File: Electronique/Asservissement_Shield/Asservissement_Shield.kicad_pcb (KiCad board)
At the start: 2 copper layers, 49 parts, among them J1 Hall_Sensor, J2 Windings, J3 Hall_Sensor, J4 Windings, P1 encoder_2, P2 encoder_2, U1 TXS0108EPW, U2 L6235PD, U3 L6235PD

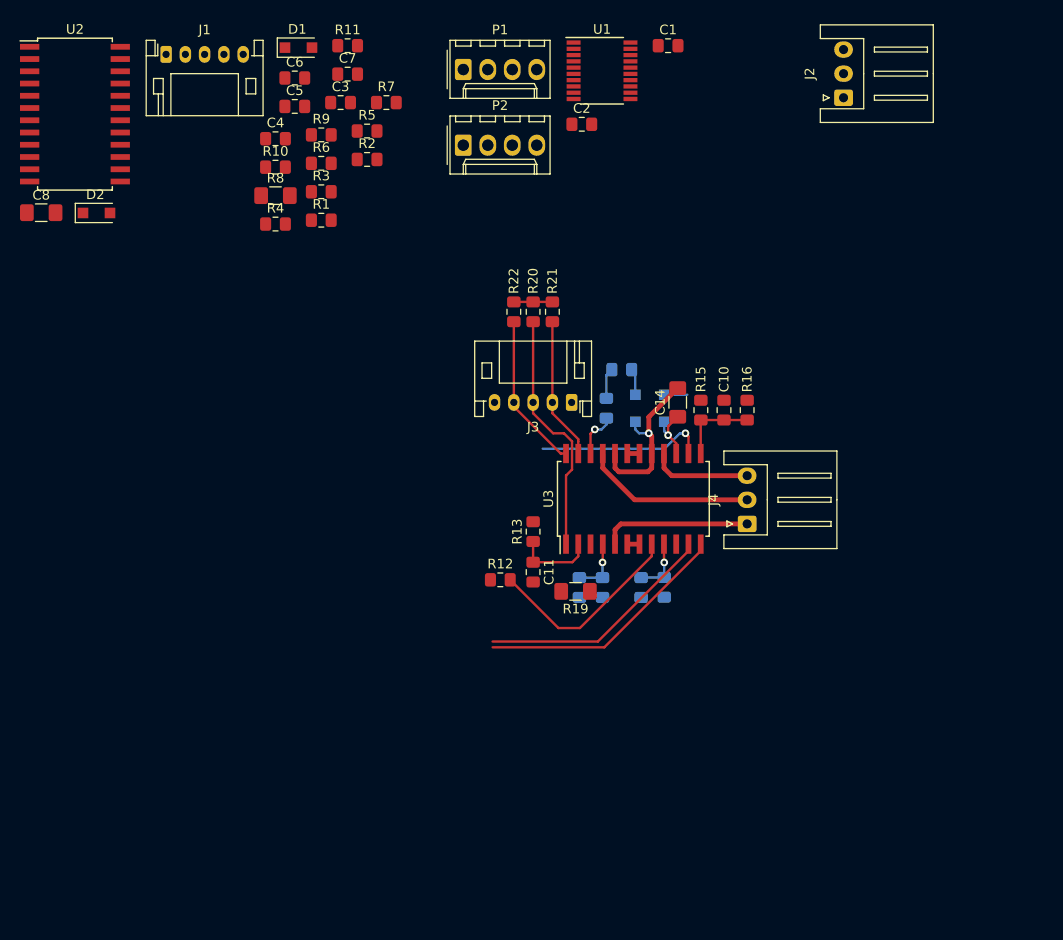
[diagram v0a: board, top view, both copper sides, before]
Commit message: oops
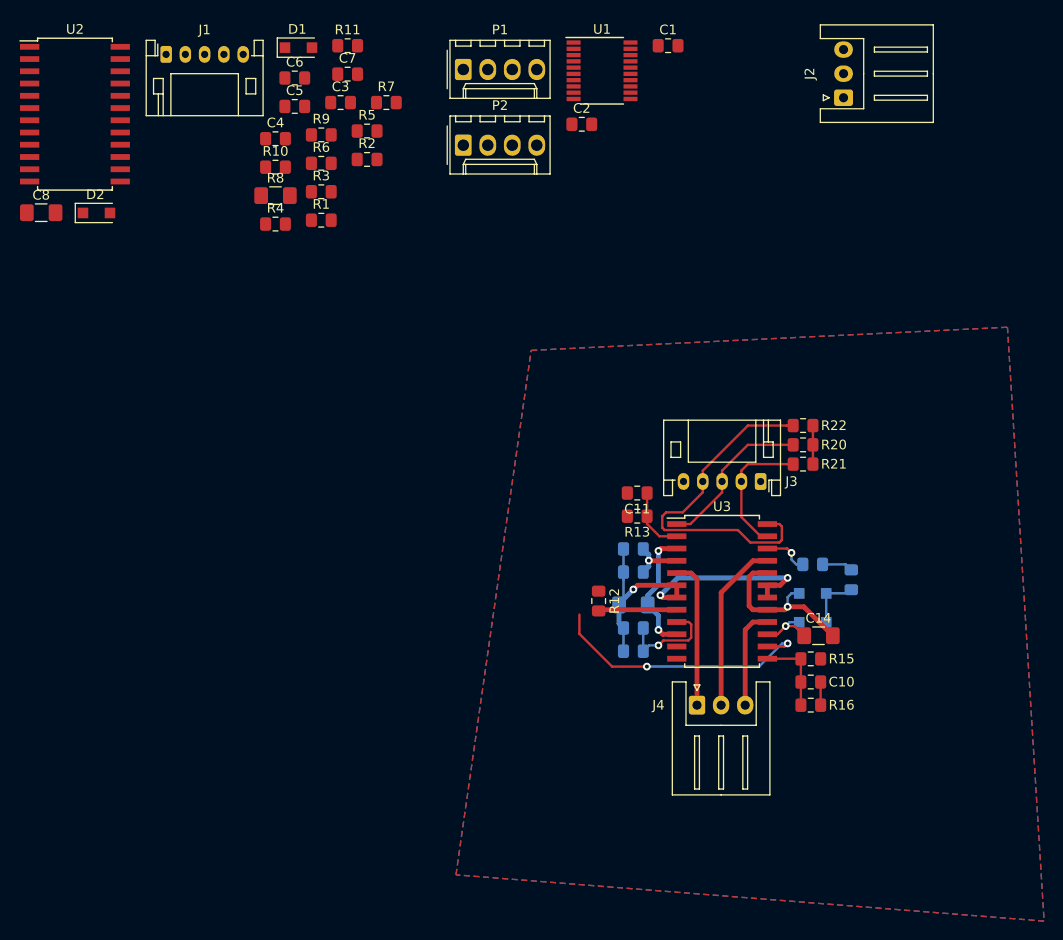
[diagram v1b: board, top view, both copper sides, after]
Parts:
- R19: moved to B.Cu
- moved C13 32.3 mm to (138.0, 91.2), turned to 90 degrees
- moved R22 32.2 mm to (133.0, 75.2), turned to 180 degrees
- moved R16 31.3 mm to (133.8, 104.2), turned to 0 degrees
- moved R20 31.2 mm to (133.0, 77.2), turned to 180 degrees
- moved R21 30.4 mm to (133.0, 79.2), turned to 180 degrees
- moved C10 29.6 mm to (133.8, 101.8), turned to 0 degrees
- moved C14 28.3 mm to (134.6, 97.0), turned to 0 degrees
- moved R15 28.2 mm to (133.8, 99.4), turned to 180 degrees
- moved D4 27.0 mm to (134.0, 95.6), turned to 0 degrees
- moved R18 26.8 mm to (134.0, 89.6), turned to 180 degrees
- moved D3 26.6 mm to (134.0, 92.6), turned to 180 degrees
- moved J3 21.2 mm to (128.6, 81.0)
- moved J4 19.5 mm to (122.0, 104.2), turned to 0 degrees
- moved C11 13.6 mm to (115.8, 82.2), turned to 180 degrees
- moved U3 13.3 mm to (124.6, 92.4), turned to 0 degrees
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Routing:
- net GND: track 2.54 -> 40.6 mm, vias 0 -> 3
- net /Diagnostic_1: track 34.8 -> 6.81 mm
- net /MotorB/Hall_Sensor3: track 16.2 -> 36.6 mm
- net (no net): track 42.6 -> 28.2 mm, vias 1 -> 2
- net Net-(R19-Pad2): track 0.00 -> 13.2 mm, vias 0 -> 2
- net /Tachometer_1: track 21.1 -> 8.15 mm
- net /MotorB/Hall_Sensor1: track 25.7 -> 16.8 mm
- net Net-(C12-Pad1): track 5.87 -> 10.9 mm
- net /MotorB/Hall_Sensor2: track 14.8 -> 14.0 mm
- added copper zone on B.Cu, net GND
- added copper zone on F.Cu, net GND
